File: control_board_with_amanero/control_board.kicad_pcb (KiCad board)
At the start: 2 copper layers, 176.3 x 196 mm, 71 parts, among them J1 Conn_Coaxial_Small, J10 Rotary Enc, J11 IR Sensor, J12 LCD, J13 DAC Board, J14 Amanero board, J16 UART to RPI4, J19 Muted out L, J2 Conn_Coaxial_Small, J20 Muted out R, J21 220vac, J3 Conn_Coaxial_Small, J4 Conn_Coaxial_Small, J9 TOS Board, K1 G6S-2, K2 G6S-2, Q1 BC547, Q2 BS170, Q3 BC547, Q4 BC547, T1 9V/10VA, T3 Triad_VPP16-310, T4 9V/10VA, U10 lt3042_breakout, U11 LT1084-ADJ, U12 LT1084-ADJ, U2 74LS573, U3 74LS573, U4 Pico, U5 ADuM1400xRW, U6 ADuM1400xRW, U7 TDR 2-1222, U8 lt3042_breakout, U9 lt3042_breakout

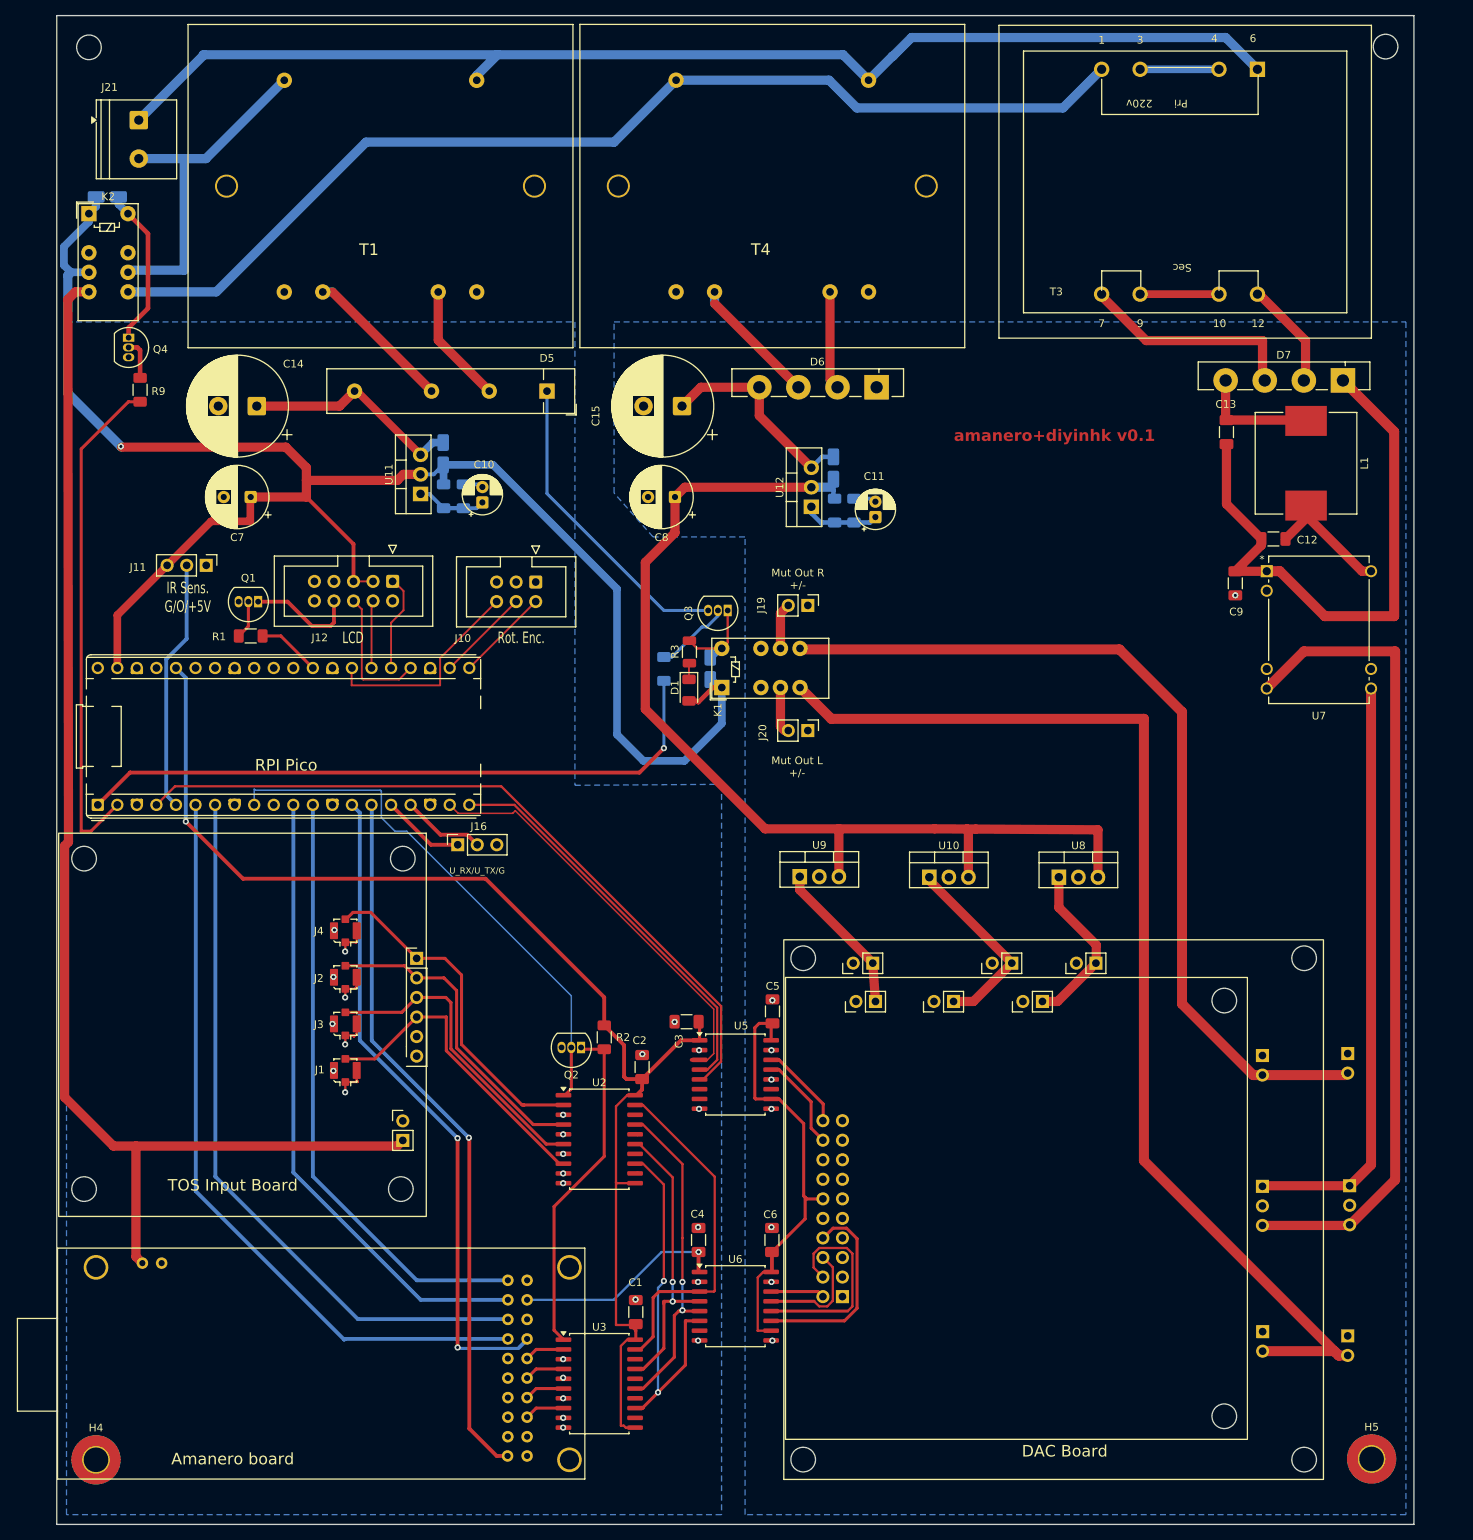
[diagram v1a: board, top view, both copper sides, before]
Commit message: v2 board
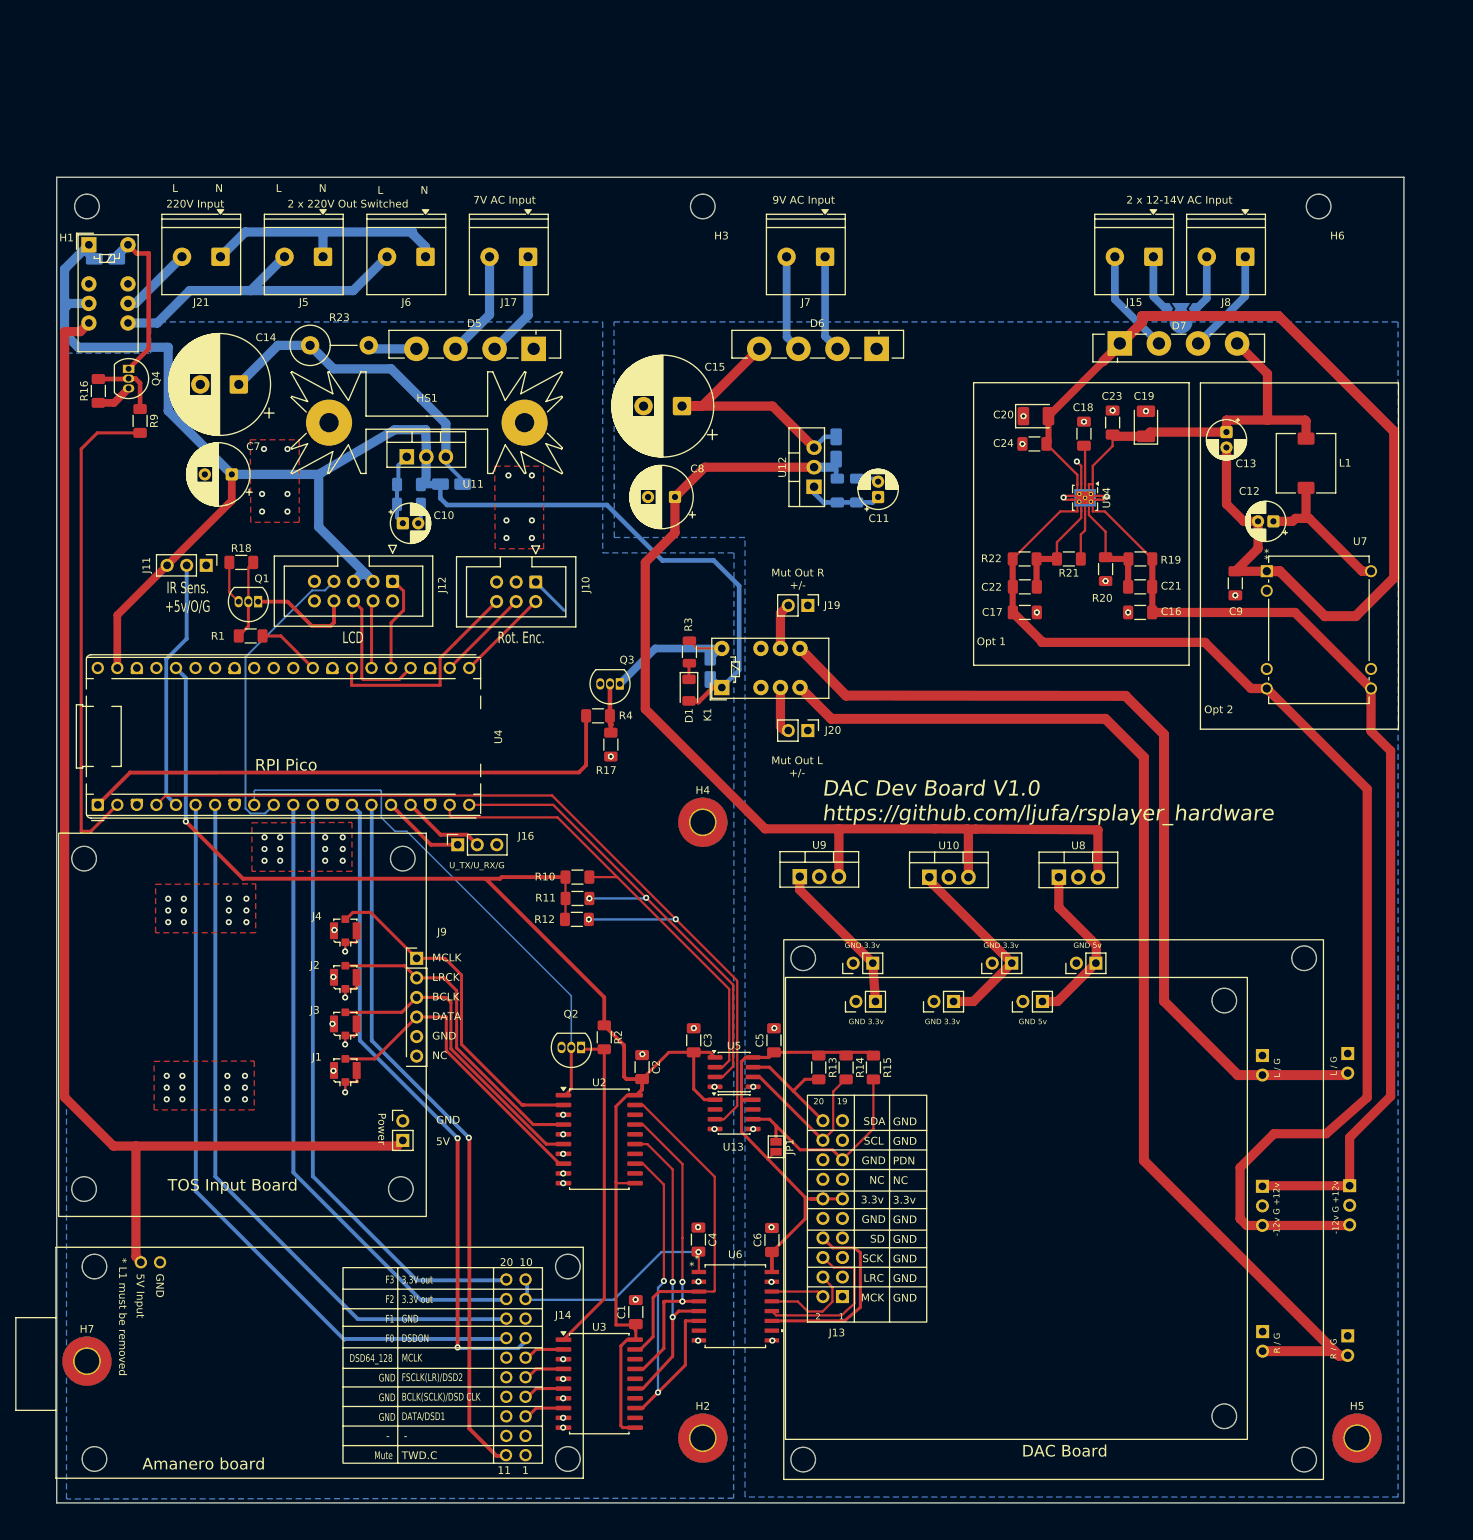
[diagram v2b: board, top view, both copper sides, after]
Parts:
- removed T1, T4: 9V/10VA, MyLibrary:MYRRA_44266
- removed T3: Triad_VPP16-310, MyLibrary:Transformer_Murata_PL10-28-130B
- added C16: Value=22uF, Capacitor_SMD:C_1206_3216Metric_Pad1.33x1.80mm_HandSolder, F.Cu at (216.9, 262.5)
- added C17: Value=22uF, Capacitor_SMD:C_1206_3216Metric_Pad1.33x1.80mm_HandSolder, F.Cu at (202.0, 262.5)
- added C18: Value=10nF, Capacitor_SMD:C_1206_3216Metric_Pad1.33x1.80mm_HandSolder, F.Cu at (209.6, 239.3)
- added C19: Value=33uF Rser=350m, Capacitor_Tantalum_SMD:CP_EIA-3528-21_Kemet-B_HandSolder, F.Cu at (217.7, 238.0)
- added C20: Value=33uF Rser=350m, Capacitor_Tantalum_SMD:CP_EIA-3528-21_Kemet-B_HandSolder, F.Cu at (203.4, 237.0)
- added C21: 0.1u, Capacitor_SMD:C_1206_3216Metric_Pad1.33x1.80mm_HandSolder, F.Cu at (216.9, 259.2)
- added C22: 0.1u, Capacitor_SMD:C_1206_3216Metric_Pad1.33x1.80mm_HandSolder, F.Cu at (202.0, 259.2)
- added C23: 0.1u, Capacitor_SMD:C_1206_3216Metric_Pad1.33x1.80mm_HandSolder, F.Cu at (213.4, 237.9)
- added C24: 0.1u, Capacitor_SMD:C_1206_3216Metric_Pad1.33x1.80mm_HandSolder, F.Cu at (203.2, 240.6)
- added H1: MountingHole, MountingHole:MountingHole_3.2mm_M3, F.Cu at (80.1, 209.8)
- added H2: GND3, MountingHole:MountingHole_3.2mm_M3_Pad_TopBottom, F.Cu at (160.1, 369.8)
- added H7: GND, MountingHole:MountingHole_3.2mm_M3_Pad_TopBottom, F.Cu at (80.1, 359.8)
- added HS1: Heatsink, Heatsink:Heatsink_Fischer_SK104-STC-STIC_35x13mm_2xDrill2.5mm, F.Cu at (124.3, 237.9)
- added J15: SEC, TerminalBlock_Philmore:TerminalBlock_Philmore_TB132_1x02_P5.00mm_Horizontal, F.Cu at (218.7, 216.3)
- added J17: SEC, TerminalBlock_Philmore:TerminalBlock_Philmore_TB132_1x02_P5.00mm_Horizontal, F.Cu at (137.4, 216.3)
- added J5: 220vac, TerminalBlock_Philmore:TerminalBlock_Philmore_TB132_1x02_P5.00mm_Horizontal, F.Cu at (110.8, 216.3)
- added J6: 220vac, TerminalBlock_Philmore:TerminalBlock_Philmore_TB132_1x02_P5.00mm_Horizontal, F.Cu at (124.1, 216.3)
- added J7: SEC, TerminalBlock_Philmore:TerminalBlock_Philmore_TB132_1x02_P5.00mm_Horizontal, F.Cu at (176.0, 216.3)
- added J8: SEC, TerminalBlock_Philmore:TerminalBlock_Philmore_TB132_1x02_P5.00mm_Horizontal, F.Cu at (230.6, 216.3)
- added JP1: open_if_u13_installed, Jumper:SolderJumper-2_P1.3mm_Open_Pad1.0x1.5mm, F.Cu at (169.6, 331.9)
- added JP4: SolderJumper_3_Open, Jumper:SolderJumper-3_P2.0mm_Open_TrianglePad1.0x1.5mm_NumberLabels, B.Cu at (222.2, 223.1)
- added R10: 10K, Resistor_SMD:R_1206_3216Metric_Pad1.30x1.75mm_HandSolder, F.Cu at (143.8, 296.9)
- added R11: 10K, Resistor_SMD:R_1206_3216Metric_Pad1.30x1.75mm_HandSolder, F.Cu at (143.8, 299.7)
- added R12: 10K, Resistor_SMD:R_1206_3216Metric_Pad1.30x1.75mm_HandSolder, F.Cu at (143.8, 302.4)
- added R13: 10K, Resistor_SMD:R_1206_3216Metric_Pad1.30x1.75mm_HandSolder, F.Cu at (175.2, 321.6)
- added R14: 10K, Resistor_SMD:R_1206_3216Metric_Pad1.30x1.75mm_HandSolder, F.Cu at (178.7, 321.6)
- added R15: 10K, Resistor_SMD:R_1206_3216Metric_Pad1.30x1.75mm_HandSolder, F.Cu at (182.3, 321.6)
- added R16: 10K, Resistor_SMD:R_1206_3216Metric_Pad1.30x1.75mm_HandSolder, F.Cu at (81.6, 233.8)
- added R17: 10K, Resistor_SMD:R_1206_3216Metric_Pad1.30x1.75mm_HandSolder, F.Cu at (148.2, 279.7)
- added R18: 10K, Resistor_SMD:R_1206_3216Metric_Pad1.30x1.75mm_HandSolder, F.Cu at (100.2, 256.0)
- added R19: 90.9K, Resistor_SMD:R_1206_3216Metric_Pad1.30x1.75mm_HandSolder, F.Cu at (217.0, 255.6)
- added R20: 10k, Resistor_SMD:R_1206_3216Metric_Pad1.30x1.75mm_HandSolder, F.Cu at (212.4, 256.9)
- added R21: 10k, Resistor_SMD:R_1206_3216Metric_Pad1.30x1.75mm_HandSolder, F.Cu at (207.7, 255.6)
- added R22: 100k, Resistor_SMD:R_1206_3216Metric_Pad1.30x1.75mm_HandSolder, F.Cu at (201.9, 255.6)
- added R23: R_Small, Resistor_THT:R_Axial_DIN0516_L15.5mm_D5.0mm_P7.62mm_Vertical, F.Cu at (109.1, 227.8)
- added U13: ADuM1250, Package_SO:SOIC-8_3.9x4.9mm_P1.27mm, F.Cu at (164.2, 327.7)
- added U14: TPS7A39, Package_SON:Texas_S-PVSON-N10_ThermalVias, F.Cu at (209.8, 247.6)
- C11: value C_Polarized -> 10uF
- C12, C13: footprint Capacitor_SMD:C_1206_3216Metric_Pad1.33x1.80mm_HandSolder -> Capacitor_THT:CP_Radial_D5.0mm_P2.00mm
- C14: value 1000uF -> 470uF
- C15: value C_Polarized -> 470uF
- C8: value C_Polarized -> 100uF
- D5: footprint Diode_THT:Diode_Bridge_32.0x5.6x17.0mm_P10.0mm_P7.5mm -> Diode_THT:Diode_Bridge_Vishay_GBU
- H4: value MountingHole -> GND
- H5: value MountingHole -> GND3
- L1: footprint Inductor_SMD:L_Neosid_SM-NE127_HandSoldering -> Inductor_SMD:L_SXN_SMDRI73
- R1, R9: value R -> 1K
- R2: value R -> 10K
- R4: value R -> 1K; moved to F.Cu
- R5, R6: value R -> 100
- R7: value R_Small -> 300
- R8: value R_Small -> 470
- U2, U3: value 74LS573 -> 74AC573
- U5: value ADuM1400xRW -> ADuM1250; footprint Package_SO:SOIC-16W_7.5x10.3mm_P1.27mm -> Package_SO:SOIC-8_3.9x4.9mm_P1.27mm
- U6: value ADuM1400xRW -> IL715E; footprint Package_SO:SOIC-16W_7.5x10.3mm_P1.27mm -> MyLibrary:SOIC16_WIDE_NVE
- U7: value TDR 2-1222 -> TDR 2-2422
- moved H4 114.3 mm to (160.1, 289.8)
- moved H3 82.4 mm to (160.1, 209.8)
- moved D7 29.4 mm to (214.3, 227.6), turned to 0 degrees
- moved H6 22.5 mm to (240.1, 209.8)
- moved J21 20.7 mm to (97.5, 216.3), turned to 180 degrees
- moved Q3 17.0 mm to (149.3, 271.8)
- moved C10 10.7 mm to (121.2, 251.0), turned to 0 degrees
- moved R4 10.5 mm to (146.5, 276.0), turned to 0 degrees
- moved D8 8.06 mm to (82.5, 216.6)
- moved R7 7.15 mm to (122.0, 248.5), turned to 0 degrees
- moved D5 5.76 mm to (138.2, 228.3)
- moved U11 5.14 mm to (121.7, 242.3), turned to 0 degrees
- moved D6 4.99 mm to (182.7, 228.3)
- moved R5 4.75 mm to (122.0, 245.9), turned to 0 degrees
- moved D3 4.09 mm to (127.5, 245.9), turned to 180 degrees
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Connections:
- net /psu/220VAC_Raw_1 renamed /psu/220_L_RAW
- net Net-(J12-Pin_8) renamed /LCD_BLK_GND
- C3 pad 1: /PICO_3.3V_OUT -> GND
- C3 pad 2: GND -> /PICO_3.3V_OUT
- C4 pad 1: /AMANERO_3.3V_OUT -> GND
- C4 pad 2: GND -> /AMANERO_3.3V_OUT
- D5 pad 4: Net-(D3-K) -> Net-(D5-+)
- J12 pad 10: unconnected-(J12-Pin_10-Pad10) -> GND
- J12 pad 7: unconnected-(J12-Pin_7-Pad7) -> /LCD_SPI_RS/DC
- J12 pad 9: unconnected-(J12-Pin_9-Pad9) -> GND
- J13 pad 11: unconnected-(J13-Pin_11-Pad11) -> /DAC_3.3V_OUT
- J13 pad 15: unconnected-(J13-Pin_15-Pad15) -> /DAC_PDN_CTRL_ISO
- J14 pad 10: unconnected-(J14-Pin_10-Pad10) -> /AMANERO_3.3V_OUT
- J14 pad 4: /DAC_I2S_LR_B -> /DAC_I2S_SCK_B
- J14 pad 5: /DAC_I2S_SCK_B -> /DAC_I2S_LR_B
- J21 pad 1: /psu/220VAC_Raw_2 -> /psu/220_N
- K2 pad 8: Net-(T4-AA) -> /psu/220_L_SWITCHED
- U3 pad 15: /DAC_I2S_LR -> /DAC_I2S_SCK
- U3 pad 17: /DAC_I2S_SCK -> /DAC_I2S_LR
- U3 pad 4: /DAC_I2S_SCK_B -> /DAC_I2S_LR_B
- U3 pad 6: /DAC_I2S_LR_B -> /DAC_I2S_SCK_B
- U4 pad 10: unconnected-(U4-GPIO7-Pad10) -> /LCD_SPI_RS/DC
- U5 pad 2: GND -> /DAC_I2C_SDA
- U5 pad 3: /DAC_I2C_SDA -> /DAC_I2C_SCL
- U5 pad 4: /DAC_I2C_SCL -> GND
- U5 pad 5: /DAC_PDN_CTRL -> GND3
- U5 pad 6: unconnected-(U5-VID-Pad6) -> /DAC_I2C_SCL_ISO
- U5 pad 7: unconnected-(U5-NC-Pad7) -> /DAC_I2C_SDA_ISO
- U5 pad 8: GND -> /DAC_3.3V_OUT
- U6 pad 10: /DAC_3.3V_OUT -> unconnected-(U6-NC-Pad10)
- U6 pad 12: /DAC_I2S_LR_ISO -> /DAC_I2S_SCK_ISO
- U6 pad 13: /DAC_I2S_SCK_ISO -> /DAC_I2S_LR_ISO
- U6 pad 4: /DAC_I2S_SCK -> /DAC_I2S_LR
- U6 pad 5: /DAC_I2S_LR -> /DAC_I2S_SCK
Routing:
- net /psu/220VAC_Raw_2: track 158.8 -> 0.00 mm
- net Net-(T4-AA): track 141.4 -> 0.00 mm
- net Net-(D7--): track 76.2 -> 131.8 mm
- net +12V: track 77.4 -> 129.3 mm
- net -12V: track 107.0 -> 155.0 mm
- net /psu/220_L_SWITCHED: track 0.00 -> 43.4 mm
- net /LCD_SPI_RS/DC: track 0.00 -> 39.6 mm
- net /psu/220_L_RAW: track 45.7 -> 9.53 mm
- net /psu/220_N: track 0.00 -> 33.5 mm
- net Net-(D7-+): track 15.6 -> 49.0 mm
- net /DAC_PDN_CTRL_ISO: track 0.00 -> 28.0 mm
- net GND: track 60.0 -> 34.9 mm, vias 26 -> 75
- net /PICO_3.3V_OUT: track 166.1 -> 189.3 mm
- net /DAC_PDN_CTRL: track 97.1 -> 117.0 mm, vias 0 -> 2
- net +5V: track 222.9 -> 205.5 mm, vias 1 -> 0
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- added copper zone on F.Cu, net GND
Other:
- board size 176.3 x 196 mm -> 175 x 172.2 mm
- board text added: "2 x 12-14V AC Input"
- board text added: "2 x 220V Out Switched"
- board text added: "220V Input"
- board text added: "7V AC Input"
- board text added: "9V AC Input"
- board text added: "DAC Dev Board V1.0 https://github.com/ljufa/rsplayer_hardware"
- board text added: "IR Sens. +5v/O/G"
- board text added: "L"
- board text added: "N"
- board text added: "Opt 1"
- board text added: "Opt 2"
- board text added: "Psu OPT1 only dual secondaries: - JP4 Short 1-2-3 Psu OPT2 dual secondaries: - JP4 1-3 short"
- board text added: "U_TX/U_RX/G"
- board text removed: "IR Sens. G/O/+5V"
- board text removed: "U_RX/U_TX/G"
- board text removed: "amanero+diyinhk v0.1"
